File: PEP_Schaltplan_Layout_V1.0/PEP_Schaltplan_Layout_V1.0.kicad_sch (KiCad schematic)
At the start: 60 parts, among them J1 2N3819, Q1 2N2222, Q2 2N2907, U10 LT1818, U2 LM7805, U3 LM7905, U4 LT1818, U5 LT1818, U6 LT1818, U7 LT1818, U8 LT1818, U9 LT1818

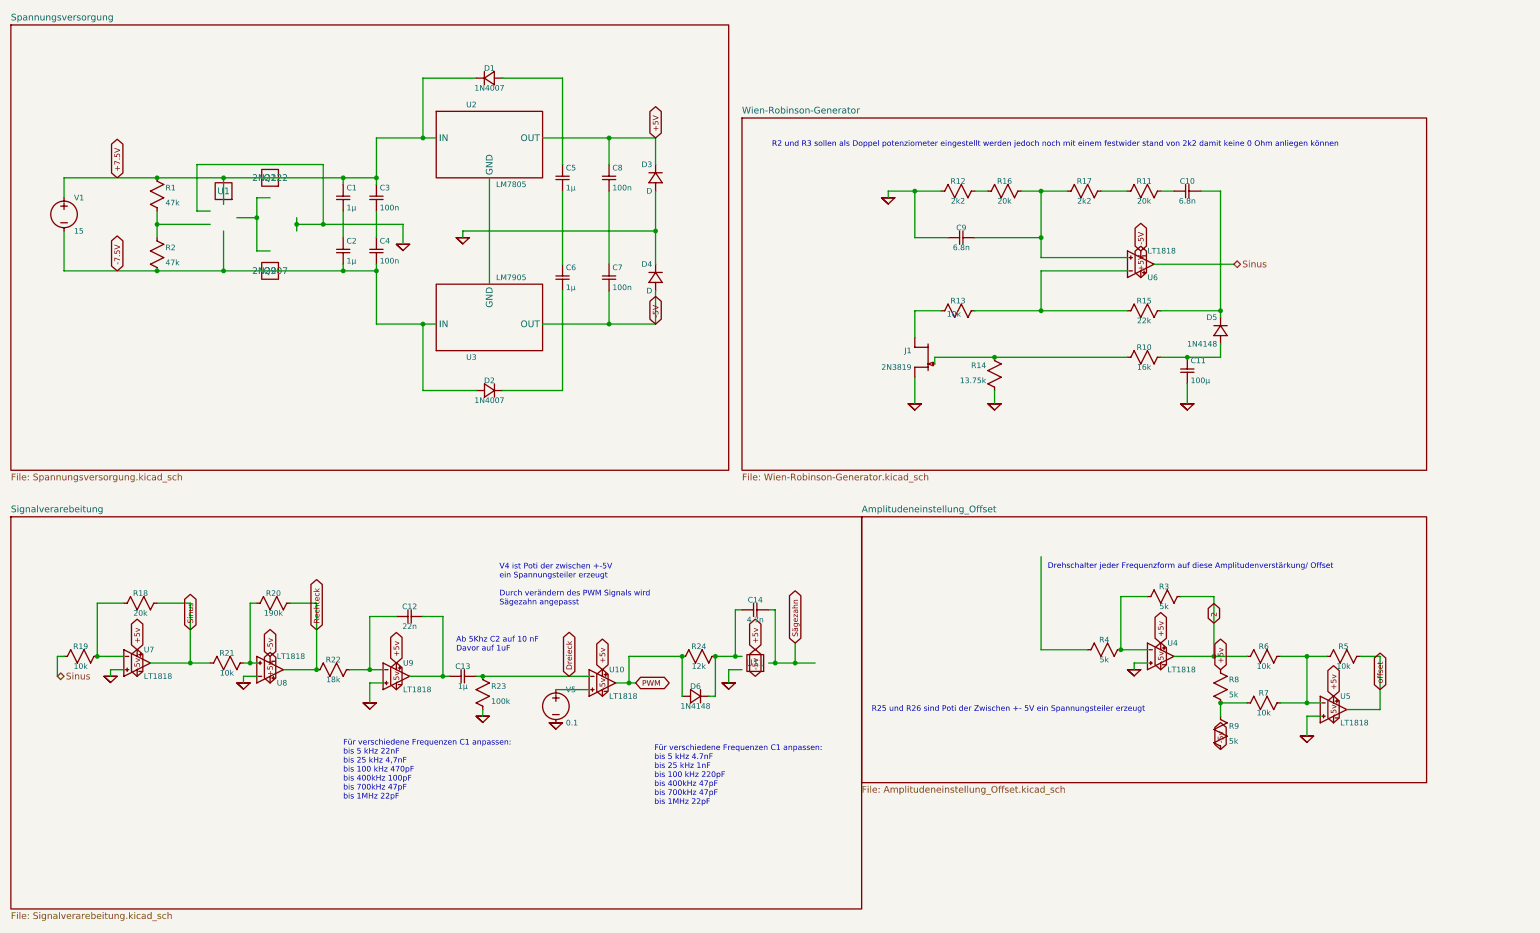
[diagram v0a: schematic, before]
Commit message: Überarbeitung und Bereinigung
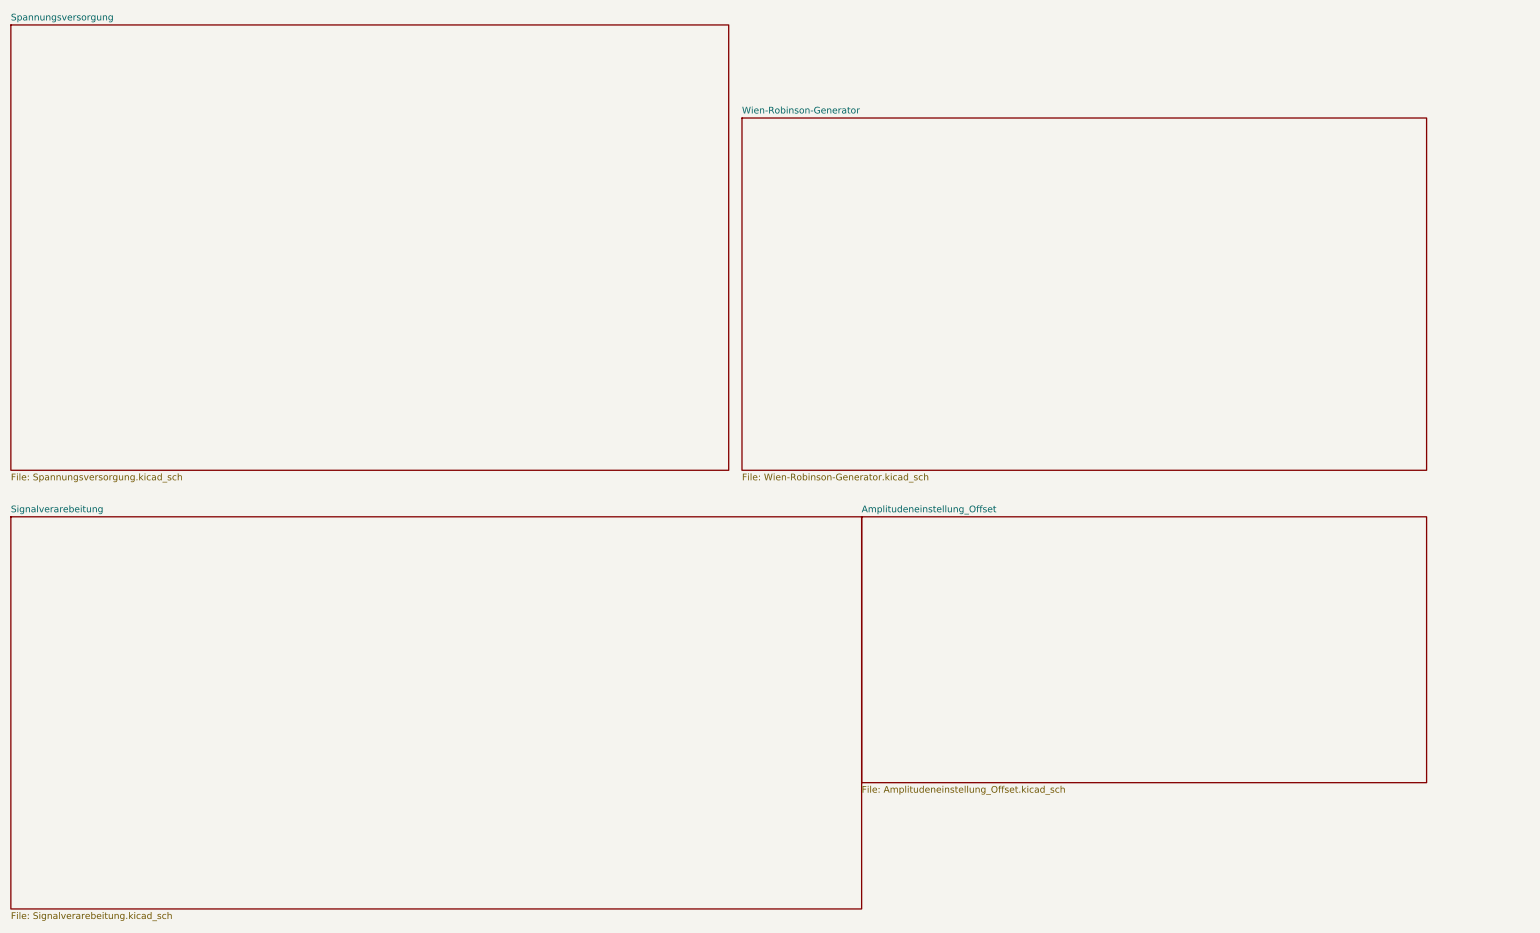
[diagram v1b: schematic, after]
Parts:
- removed C1, C13, C2, C5, C6: 1µ, symbol ltspice:cap
- removed C10, C9: 6.8n, symbol ltspice:cap
- removed C11: 100µ, symbol ltspice:cap
- removed C12: 22n, symbol ltspice:cap
- removed C14: 4.7n, symbol ltspice:cap
- removed C3, C4, C7, C8: 100n, symbol ltspice:cap
- removed D1, D2: 1N4007, symbol ltspice:diode
- removed D3, D4: D, symbol ltspice:diode
- removed D5, D6: 1N4148, symbol ltspice:diode
- removed J1: 2N3819, symbol ltspice:njf
- removed Q1: 2N2222, symbol ltspice:lib/sym/npn
- removed Q2: 2N2907, symbol ltspice:lib/sym/pnp
- removed R1, R2: 47k, symbol ltspice:res
- removed R10: 16k, symbol ltspice:res
- removed R11, R16, R18: 20k, symbol ltspice:res
- removed R12, R17: 2k2, symbol ltspice:res
- removed R13, R19, R21, R5, R6, R7: 10k, symbol ltspice:res
- removed R14: 13.75k, symbol ltspice:res
- removed R15: 22k, symbol ltspice:res
- removed R20: 190k, symbol ltspice:res
- removed R22: 18k, symbol ltspice:res
- removed R23: 100k, symbol ltspice:res
- removed R24: 12k, symbol ltspice:res
- removed R3, R4, R8, R9: 5k, symbol ltspice:res
- removed U1: (no value), symbol ltspice:lib/sym/OpAmps/LT1001
- removed U10, U4, U5, U6, U7, U8, U9: LT1818, symbol ltspice:OpAmps/LT1818
- removed U11: (no value), symbol ltspice:lib/sym/OpAmps/LT1819
- removed U2: LM7805, symbol ltspice:7805
- removed U3: LM7905, symbol ltspice:7905
- removed V1: 15, symbol ltspice:voltage
- removed V5: 0.1, symbol ltspice:voltage
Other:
- note removed: "Ab 5Khz C2 auf 10 nF Davor auf 1uF"
- note removed: "Drehschalter jeder Frequenzform auf diese Amplitudenverstärkung/ Offset"
- note removed: "Für verschiedene Frequenzen C1 anpassen: bis 5 kHz 22nF bis 25 kHz 4,7nF bis 100 kHz 470pF bis 400kHz 100pF bis 700kHz 47pF bis 1MHz 22pF"
- note removed: "Für verschiedene Frequenzen C1 anpassen: bis 5 kHz 4.7nF bis 25 kHz 1nF bis 100 kHz 220pF bis 400kHz 47pF bis 700kHz 47pF bis 1MHz 22pF"
- note removed: "R2 und R3 sollen als Doppel potenziometer eingestellt werden jedoch noch mit einem festwider stand von 2k2 damit keine 0 Ohm anliegen können"
- note removed: "R25 und R26 sind Poti der Zwischen +- 5V ein Spannungsteiler erzeugt"
- note removed: "V4 ist Poti der zwischen +-5V ein Spannungsteiler erzeugt Durch verändern des PWM Signals wird Sägezahn angepasst"
